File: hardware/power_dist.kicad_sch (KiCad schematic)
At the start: 15 parts, among them U7 LT1962-3.3, U8 TPS62177DQC

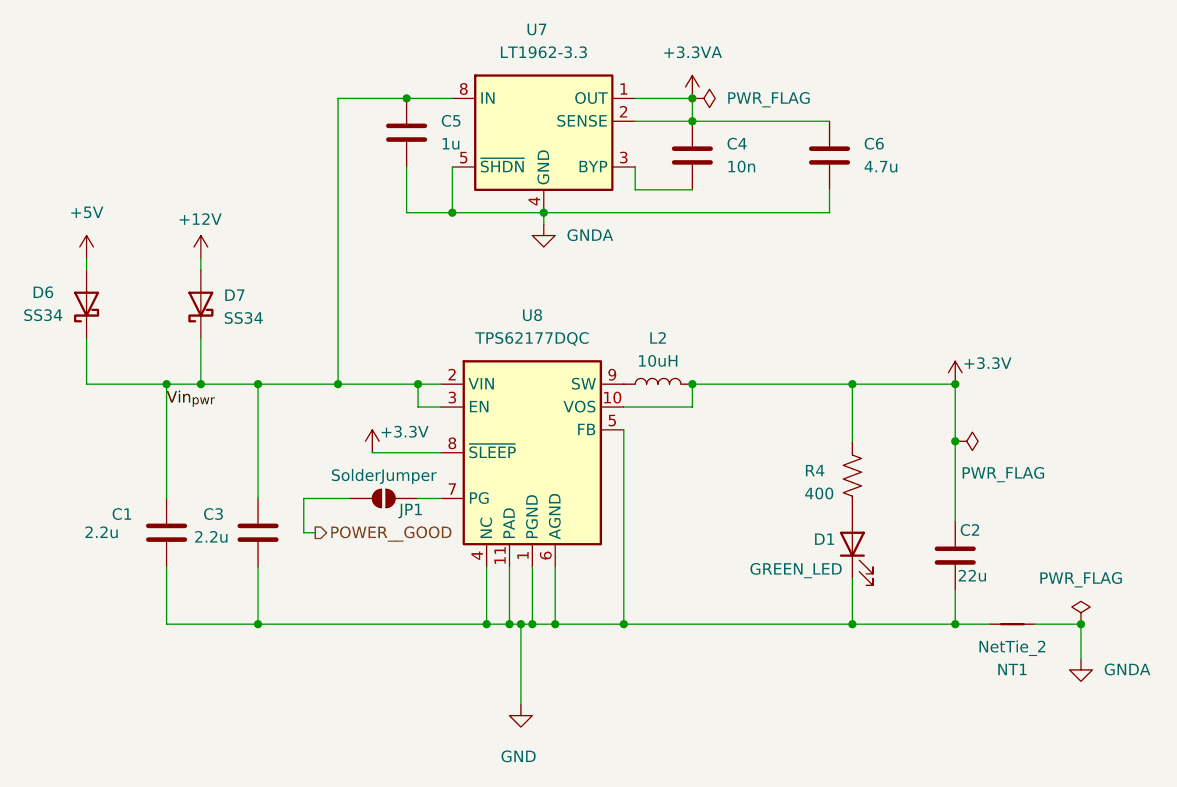
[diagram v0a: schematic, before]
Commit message: adding overdue changes
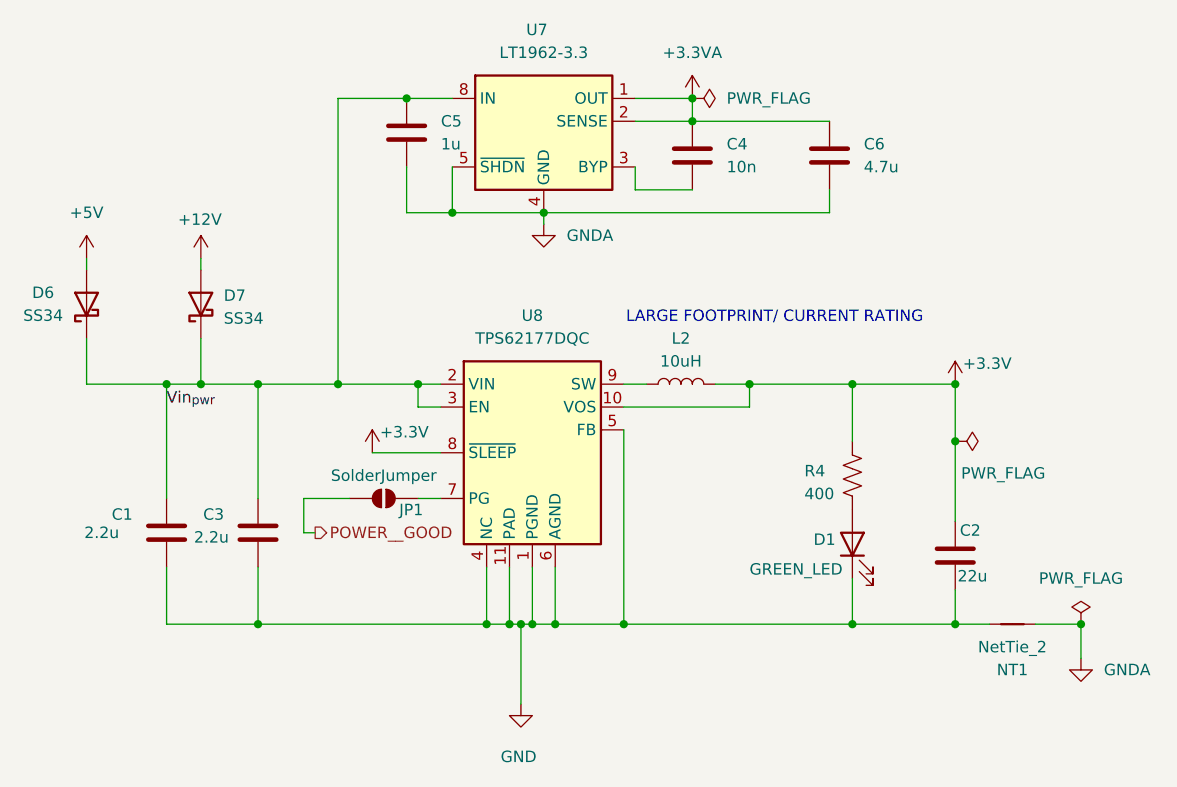
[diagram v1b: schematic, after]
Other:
- note added: "LARGE FOOTPRINT/ CURRENT RATING"
- moved on the sheet: L2
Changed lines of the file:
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@@
 		(company "University of Toronto Human Powered Vehicles")
 	)
+	(text "LARGE FOOTPRINT/ CURRENT RATING"
+		(exclude_from_sim no)
+		(at 133.604 51.054 0)
+		(effects
+			(font
+				(size 1.27 1.27)
+			)
+		)
+	)
+	(junction
+		(at 130.81 58.42)
+		(diameter 0)
+		(color 0 0 0 0)
+	)
 	(junction
 		(at 104.14 85.09)
@@
 	)
 	(junction
-		(at 124.46 58.42)
-		(diameter 0)
-		(color 0 0 0 0)
-	)
-	(junction
 		(at 167.64 85.09)
 		(diameter 0)
@@
 	(wire
 		(pts
-			(xy 124.46 58.42) (xy 142.24 58.42)
+			(xy 127 58.42) (xy 130.81 58.42)
 		)
 		(stroke
@@
 	(wire
 		(pts
+			(xy 130.81 58.42) (xy 142.24 58.42)
+		)
+		(stroke
+			(width 0)
+			(type default)
+		)
+	)
+	(wire
+		(pts
 			(xy 66.04 78.74) (xy 66.04 85.09)
 		)
@@
 	(wire
 		(pts
-			(xy 116.84 60.96) (xy 124.46 60.96)
+			(xy 116.84 60.96) (xy 130.81 60.96)
 		)
 		(stroke
@@
 	(wire
 		(pts
-			(xy 124.46 60.96) (xy 124.46 58.42)
+			(xy 130.81 60.96) (xy 130.81 58.42)
 		)
 		(stroke
@@
 		(pts
 			(xy 82.55 74.93) (xy 81.28 74.93)
+		)
+		(stroke
+			(width 0)
+			(type default)
+		)
+	)
+	(wire
+		(pts
+			(xy 119.38 58.42) (xy 116.84 58.42)
 		)
 		(stroke
@@
 	(symbol
 		(lib_id "Device:L")
-		(at 120.65 58.42 90)
+		(at 123.19 58.42 90)
 		(unit 1)
 		(exclude_from_sim no)
@@
 		(fields_autoplaced yes)
 		(property "Reference" "L2"
-			(at 120.65 53.34 90)
+			(at 123.19 53.34 90)
 			(effects
 				(font
@@
 		)
 		(property "Value" "10uH"
-			(at 120.65 55.88 90)
+			(at 123.19 55.88 90)
 			(effects
 				(font
@@
 		)
 		(property "Footprint" "Inductor_SMD:L_0603_1608Metric"
-			(at 120.65 58.42 0)
+			(at 123.19 58.42 0)
 			(effects
 				(font
@@
 		)
 		(property "Datasheet" "~"
-			(at 120.65 58.42 0)
+			(at 123.19 58.42 0)
 			(effects
 				(font
@@
 		)
 		(property "Description" "Inductor"
-			(at 120.65 58.42 0)
+			(at 123.19 58.42 0)
 			(effects
 				(font
@@
 		)
 		(property "LCSC" "C86083"
-			(at 120.65 58.42 90)
-			(effects
-				(font
+			(at 123.19 58.42 90)
+			(effects
+				(font
